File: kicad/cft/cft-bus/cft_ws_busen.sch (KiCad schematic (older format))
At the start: 40 parts, among them U22 ICS501, U34 74LVC1G32, U43 74LVC1G04, U44 74LVC1G3208, U45 74LVC1G125, U46 74AHC1G32, U47 74LVC1G74, U48 74HC245, U49 74LVC1G11, U50 74HC245, U51 74LVC1G3208, U52 74LVC1G17, U53 74LVC1G373

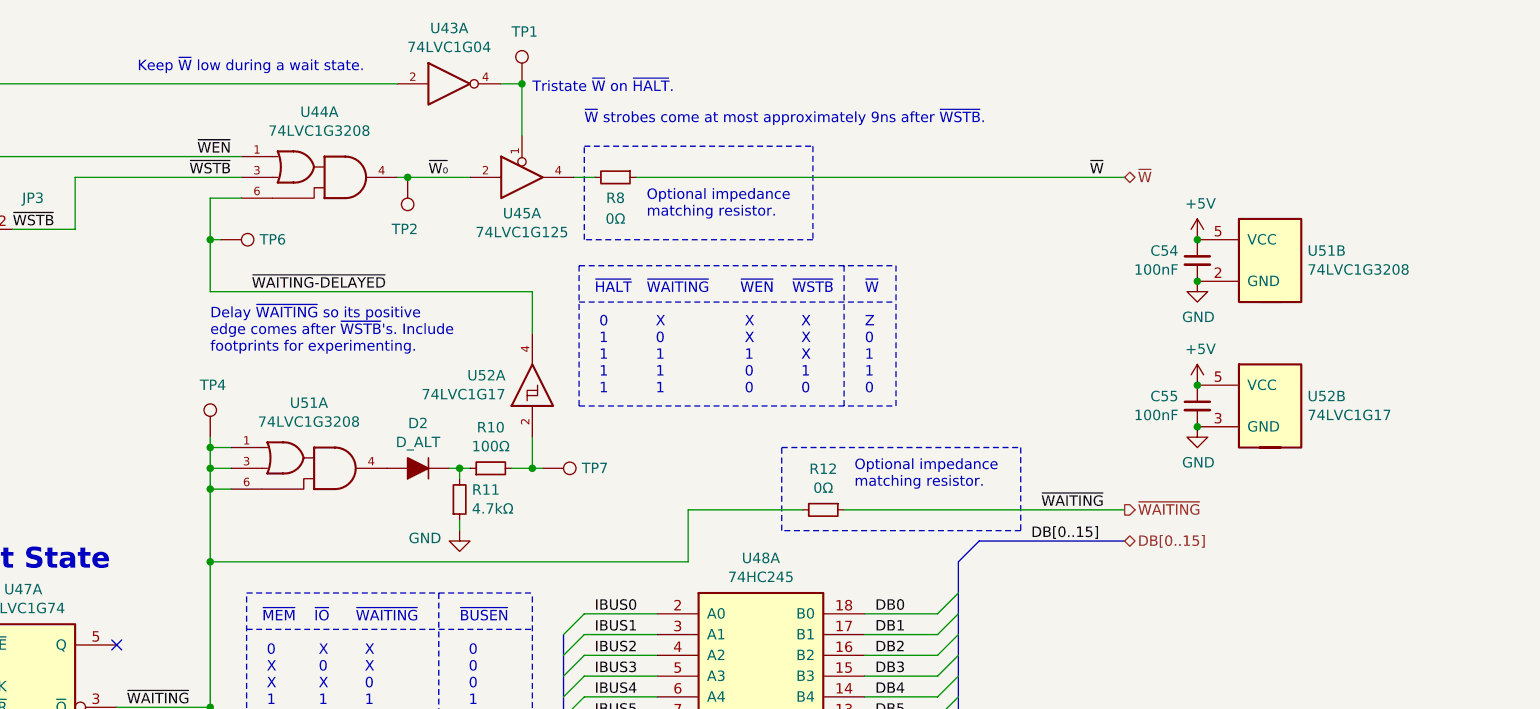
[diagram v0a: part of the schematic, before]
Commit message: Working on CTL board.
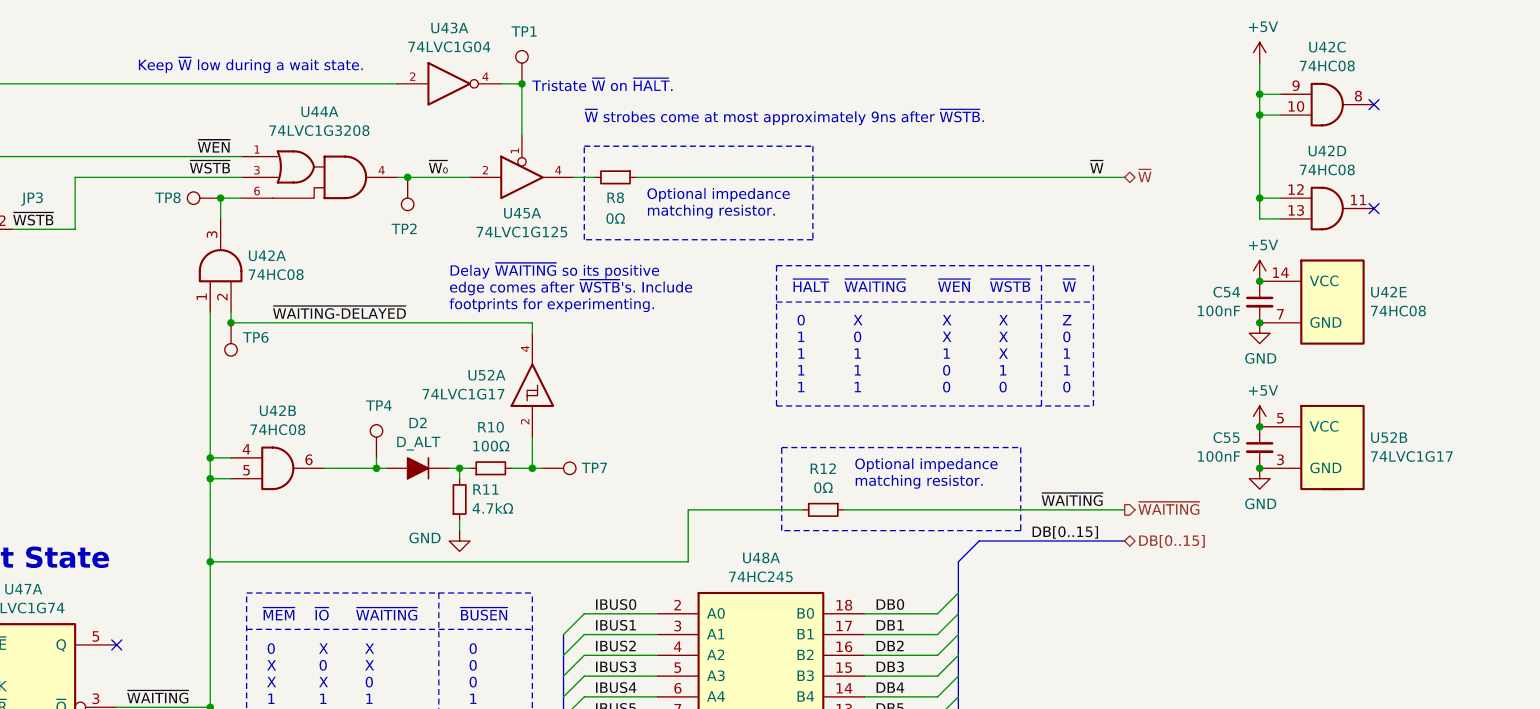
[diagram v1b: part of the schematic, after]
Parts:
- removed U51: 74LVC1G3208, alexios:SOT-23-6_Handsoldering, symbol alexios:74LVC1G3208
- added TP8: TestPoint, TestPoint:TestPoint_Pad_1.0x1.0mm, symbol Connector:TestPoint
- added U42: 74HC08, alexios:SOIC-14, symbol alexios:74HC08
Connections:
- net +5V: now also U42.10, U42.12, U42.13, U42.14 (VCC), U42.9
- net GND: now also U42.7 (GND)
- net ~WAITING: now also U42.1, U42.4, U42.5; no longer TP4.1
- net ~WAITING-DELAYED: now also U42.2; no longer U44.6
- net at D2.2 (A): now also TP4.1, U42.6
- new net: TP8.1, U42.3, U44.6
- no-connect marks 3 -> 5
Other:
- moved on the sheet: C54, C55, TP4, TP6, U52B

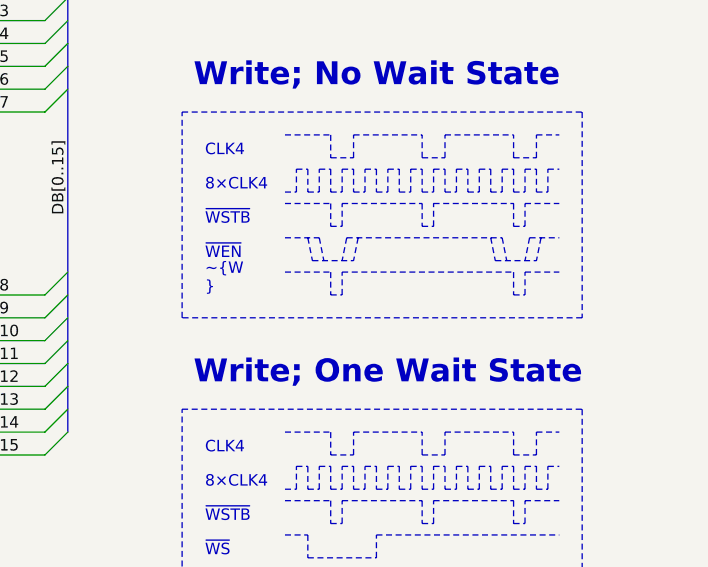
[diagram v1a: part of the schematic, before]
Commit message: Fixing serious potential processor bug by readjusting clocks and establishing standard waveforms.
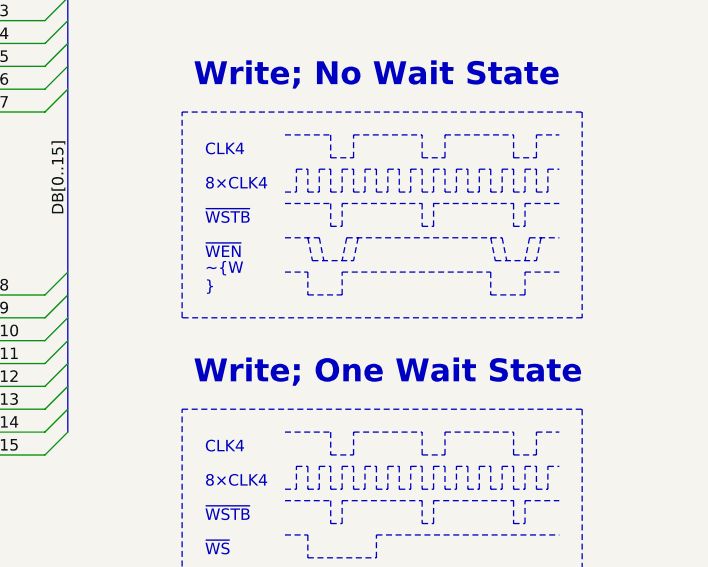
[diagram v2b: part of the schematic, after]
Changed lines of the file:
@@
 ~W\n
 Wire Notes Line width 12 style solid
-	9700 4900 9900 4900
+	9700 4900 9800 4900
 Wire Notes Line width 12 style solid
-	9900 4900 9900 5000
+	9800 4900 9800 5000
 Wire Notes Line width 12 style solid
 	9950 5000 9950 4900
 Wire Notes Line width 12 style solid
-	9900 5000 9950 5000
+	9800 5000 9950 5000
 Wire Notes Line width 12 style solid
-	10700 4900 10700 5000
+	10600 4900 10600 5000
 Wire Notes Line width 12 style solid
 	10750 5000 10750 4900
 Wire Notes Line width 12 style solid
-	10700 5000 10750 5000
+	10600 5000 10750 5000
 Wire Notes Line width 12 style solid
 	10750 4900 10900 4900
@@
 	10770 4750 10900 4750
 Wire Notes Line width 12 style solid
-	9950 4900 10700 4900
+	9950 4900 10600 4900
 Wire Notes Line width 12 style solid
 	9970 4750 10650 4750
